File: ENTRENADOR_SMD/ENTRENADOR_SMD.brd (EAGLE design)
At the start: 100 x 100.3 mm, 76 parts, among them IC1 PIC16F1939PT, SW1 TL3342F160QG/TR

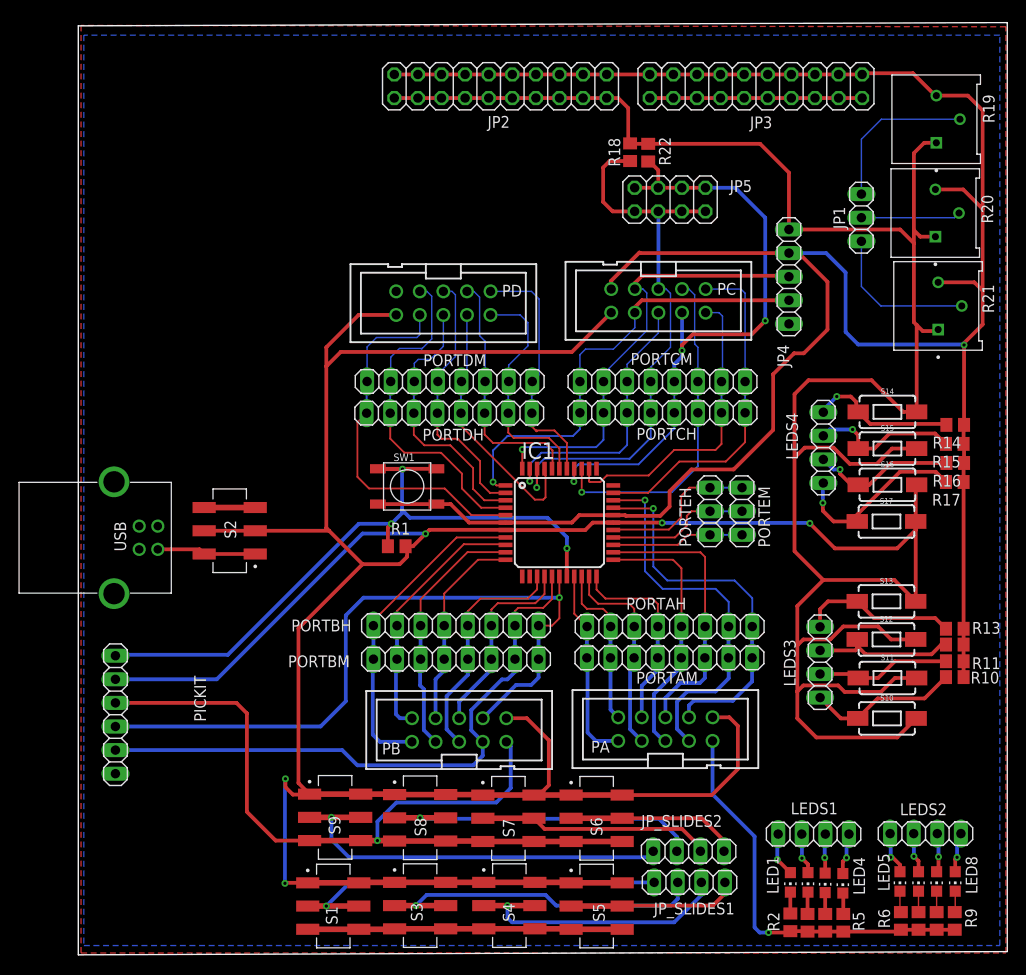
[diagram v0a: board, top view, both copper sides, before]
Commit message: Se actualiza y se argegan librerias
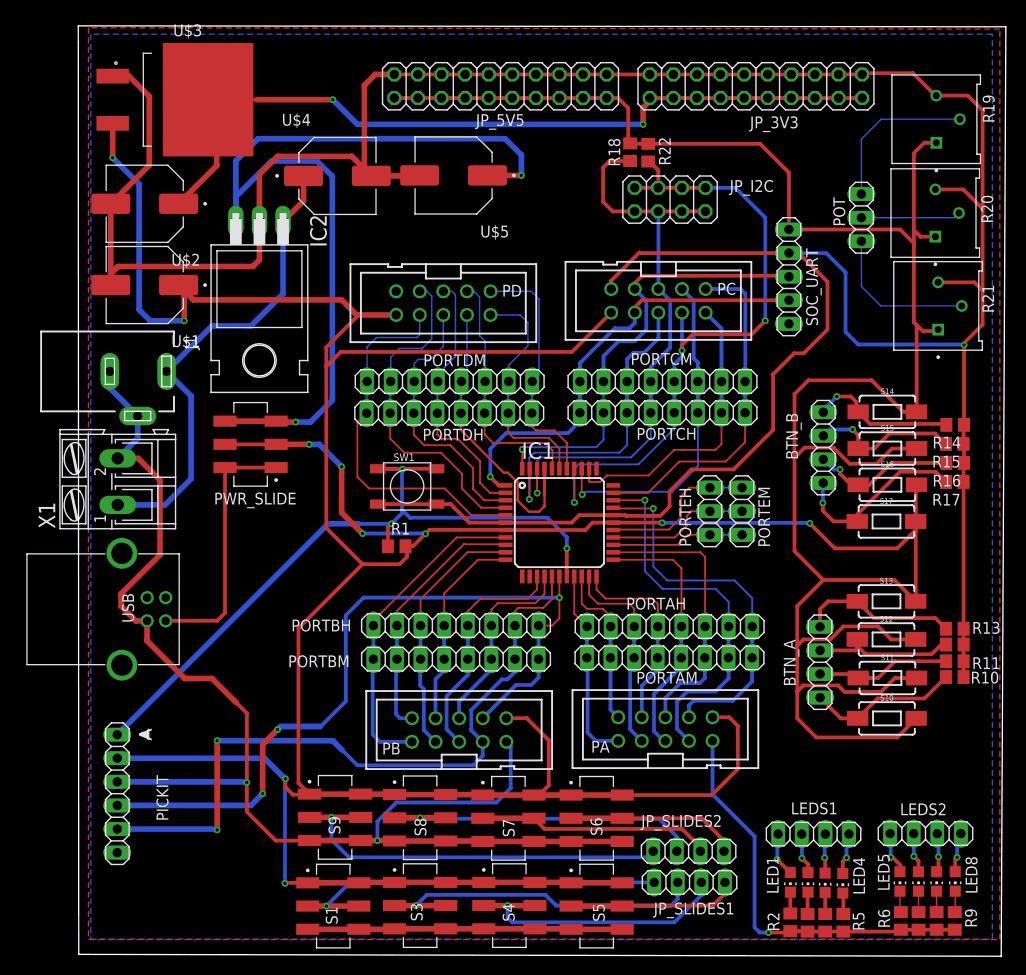
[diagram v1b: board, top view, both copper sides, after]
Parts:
- removed S2: SLDS2, JS202011SCQN:SW_JS202011SCQN
- added IC2: 7824T, linear:TO220H
- added J1: DCJ0202, con-jack:DCJ0202
- added PWR_SLIDE: SLDS2, JS202011SCQN:SW_JS202011SCQN
- added U$1, U$2, U$4, U$5: CAPA, CAPAE830X1000N:CAPA
- added U$3: VREG3V3, VREG_L7805ACD2T:VREG3V3
- added X1: (no value), con-ptr500:AK300/2
- moved PICKIT 8.50 mm to (4.20, 17.4)
- moved USB 7.75 mm to (4.70, 37.2)
- renumbered JP1 to POT, JP2 to JP_5V5, JP3 to JP_3V3, JP4 to SOC_UART, JP5 to JP_I2C, LEDS3 to BTN_A, LEDS4 to BTN_B
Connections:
- removed net GNG: PD.9
- new net N$36: IC2.1, J1.1, U$4.P, X1.1
- net 3V3: now also U$2.P, U$3.4
- net GND: now also IC2.2, J1.2, J1.3, PD.9, U$1.N, U$2.N, U$3.1, U$4.N, U$5.N, X1.2
- net VCC: now also PWR_SLIDE.2, PWR_SLIDE.5, U$1.P, U$3.3; no longer S2.2, S2.5
- net VEXT: now also IC2.3, PWR_SLIDE.3, PWR_SLIDE.6, U$5.P; no longer S2.3, S2.6
- net VUSB: now also PWR_SLIDE.1, PWR_SLIDE.4; no longer S2.1, S2.4
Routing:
- net GND: track 427.3 -> 564.2 mm, vias 3 -> 4
- net VEXT: track 5.50 -> 96.8 mm, vias 0 -> 2
- net 3V3: track 22.9 -> 87.4 mm, vias 0 -> 2
- net N$36: track 0.00 -> 51.3 mm
- net VCC: track 569.8 -> 619.2 mm, vias 5 -> 10
- net VUSB: track 10.7 -> 27.9 mm
- net RB6: track 66.0 -> 75.8 mm, vias 0 -> 2
- net RD3: track 30.2 -> 36.7 mm
- net RB7: track 79.6 -> 86.0 mm, vias 1 -> 3
- net RC5: track 30.2 -> 35.2 mm
- net RC3: track 68.7 -> 73.2 mm
- net MCLR: track 76.7 -> 80.2 mm
- net RC4: track 62.7 -> 63.7 mm
- net RC7: track 49.4 -> 48.6 mm
- net RC1: track 33.1 -> 32.3 mm
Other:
- board size 100 x 100.3 mm -> 99.8 x 100.2 mm
- board text added: "<"

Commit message: se crea diseño entrenador
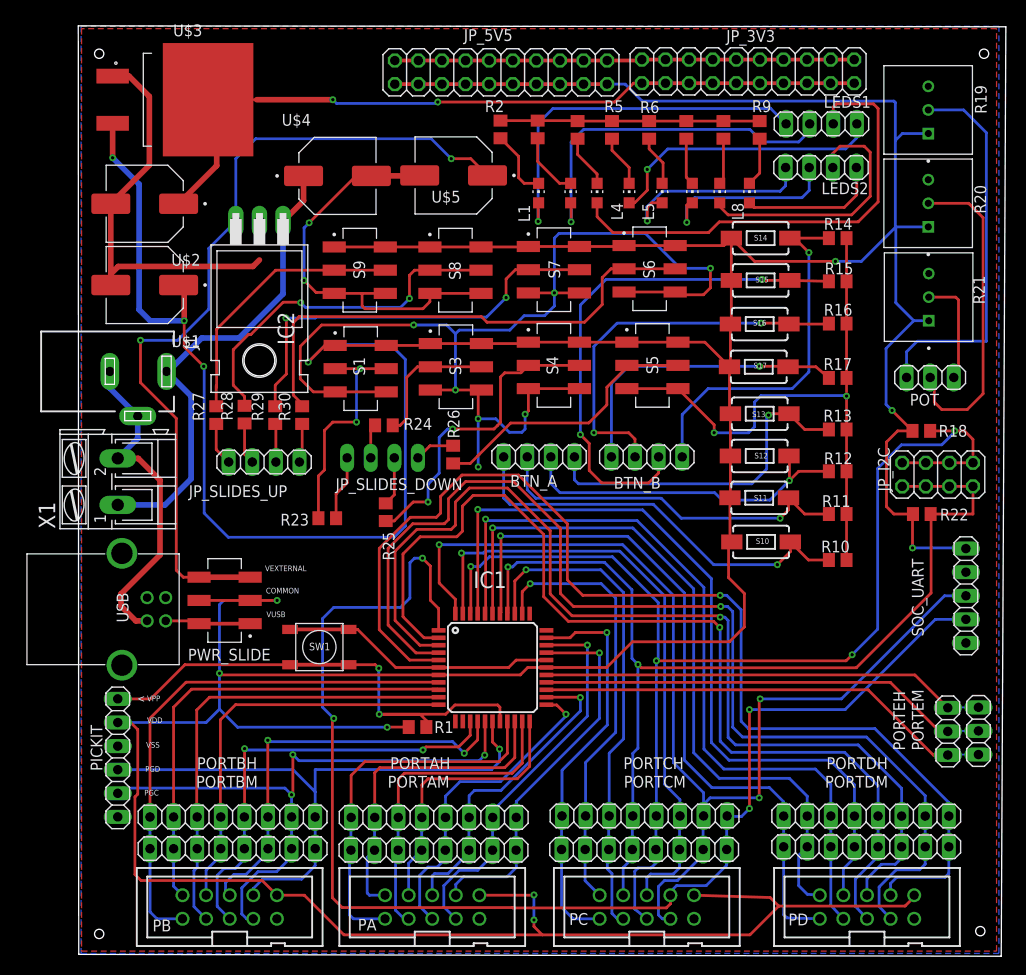
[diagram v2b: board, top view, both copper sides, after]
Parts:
- removed JP_SLIDES1, JP_SLIDES2: (no value), pinhead:1X04
- removed LED1, LED4, LED5, LED8: (no value), led:CHIP-LED0805
- added JP_SLIDES_DOWN, JP_SLIDES_UP: (no value), pinhead:1X04
- added L1, L4, L5, L8: (no value), led:CHIP-LED0805
- added R23, R24, R25, R26, R27, R28, R29, R30: 4K7, R0805_:R0805
- R1: value (none) -> 4K7
- R10, R11, R12, R13, R14, R15, R16, R17: value (none) -> 10K
- R19, R20, R21: value 3386P-1-101TLF -> COM-09806; device 3386P-1-101TLF:TRIM_3386P-1-101TLF -> COM-09806:TRIM_COM-09806
- R2, R3, R4, R5, R6, R7, R8, R9: value (none) -> 330R
- moved R2 90.9 mm to (45.5, 88.8), turned to 270 degrees
- moved R3 90.2 mm to (49.5, 88.8), turned to 270 degrees
- moved R4 89.4 mm to (53.8, 88.8), turned to 270 degrees
- moved R6 89.4 mm to (61.5, 88.8), turned to 270 degrees
- moved R5 88.9 mm to (57.5, 88.8), turned to 270 degrees
- moved R7 88.7 mm to (65.5, 88.8), turned to 270 degrees
- moved R8 88.2 mm to (69.5, 88.8), turned to 270 degrees
- moved R9 87.7 mm to (73.3, 88.8), turned to 270 degrees
- moved PD 79.4 mm to (84.9, 5.15), turned to 0 degrees
- moved LED2 78.5 mm to (53.0, 82.0), turned to 0 degrees
- moved LED3 78.2 mm to (55.9, 82.0), turned to 0 degrees
- moved LED6 78.0 mm to (66.1, 82.0), turned to 0 degrees
- moved LED7 77.7 mm to (69.0, 82.0), turned to 0 degrees
- moved LEDS1 76.5 mm to (80.0, 89.5)
- moved LEDS2 72.6 mm to (80.0, 84.8)
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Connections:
- new net N$37: JP_SLIDES_UP.1, R27.1
- new net N$38: JP_SLIDES_UP.2, R28.1
- new net N$39: JP_SLIDES_UP.3, R29.1
- new net N$40: JP_SLIDES_DOWN.1, R26.1
- new net N$41: JP_SLIDES_DOWN.2, R25.1
- new net N$42: JP_SLIDES_DOWN.3, R24.1
- new net N$43: JP_SLIDES_DOWN.4, R23.1
- new net N$44: JP_SLIDES_UP.4, R30.1
- net N$1: now also R23.2; no longer JP_SLIDES1.4
- net N$12: now also L4.C; no longer LED4.C
- net N$13: now also L5.C; no longer LED5.C
- net N$16: now also L8.C; no longer LED8.C
- net N$17: now also L1.A; no longer LED1.A
- net N$2: now also R24.2; no longer JP_SLIDES1.3
- net N$20: now also L4.A; no longer LED4.A
- net N$21: now also L5.A; no longer LED5.A
- net N$24: now also L8.A; no longer LED8.A
- net N$3: now also R25.2; no longer JP_SLIDES1.2
- net N$4: now also R26.2; no longer JP_SLIDES1.1
- net N$5: now also R30.2; no longer JP_SLIDES2.4
- net N$6: now also R29.2; no longer JP_SLIDES2.3
- net N$7: now also R28.2; no longer JP_SLIDES2.2
- net N$8: now also R27.2; no longer JP_SLIDES2.1
- net N$9: now also L1.C; no longer LED1.C
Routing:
- net GND: track 564.2 -> 420.4 mm, vias 4 -> 11
- net RC7: track 48.6 -> 146.4 mm, vias 1 -> 4
- net RD6: track 36.7 -> 119.7 mm, vias 0 -> 1
- net RD7: track 40.4 -> 122.9 mm, vias 0 -> 1
- net RD5: track 29.1 -> 110.7 mm, vias 0 -> 1
- net RD4: track 28.8 -> 106.7 mm, vias 0 -> 1
- net RC6: track 48.5 -> 119.4 mm, vias 1 -> 3
- net RC4: track 63.7 -> 132.0 mm, vias 1 -> 4
- net RD2: track 26.8 -> 84.4 mm, vias 0 -> 1
- net RD1: track 25.5 -> 78.1 mm, vias 0 -> 1
- net RD0: track 27.1 -> 77.5 mm, vias 0 -> 1
- net RD3: track 36.7 -> 86.8 mm, vias 0 -> 1
- net N$19: track 4.25 -> 50.9 mm, vias 1 -> 0
- net N$30: track 16.3 -> 56.3 mm, vias 1 -> 2
- net RC3: track 73.2 -> 112.4 mm, vias 3 -> 2
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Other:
- board text added: "COMMON"
- board text added: "VEXTERNAL"
- board text added: "VUSB"
- board text removed: "SCL"
- board text removed: "SDA"
